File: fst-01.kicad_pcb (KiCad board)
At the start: 2 copper layers, 26.5 x 13.1 mm, 24 parts, among them J1 USB_A, K1 CONN_3, K2 CONN_2, K3 CONN_2, U1 STM32F103TB, U2 LP2985-33DBVR, U3 NUF2221W1, U4 SST25VF032B, X1 12MHz

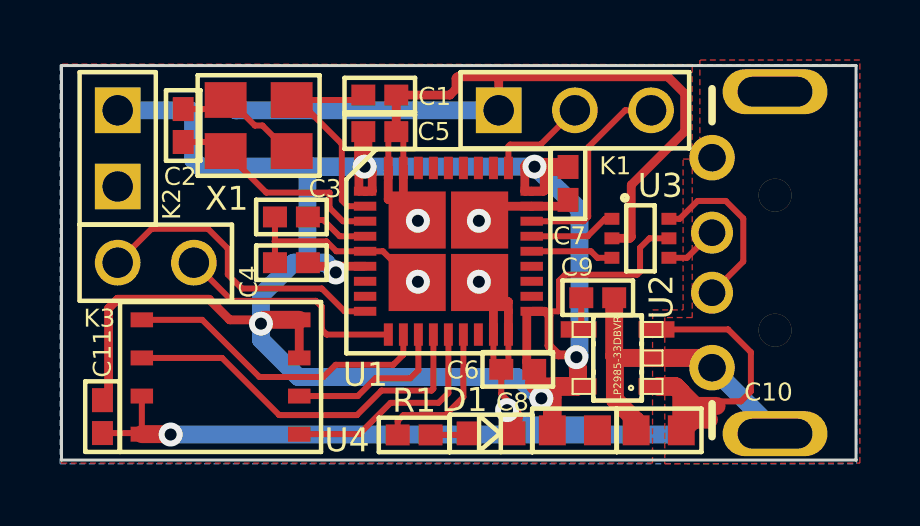
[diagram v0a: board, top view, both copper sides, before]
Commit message: update PCB
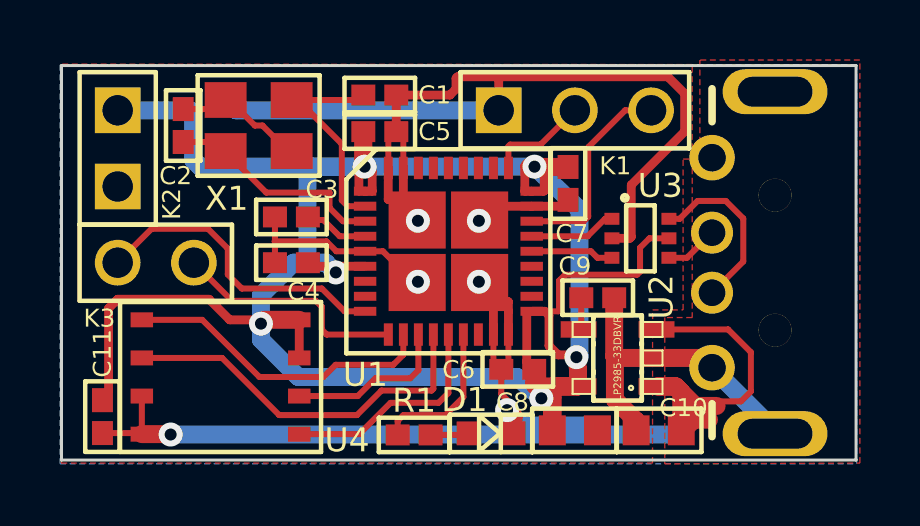
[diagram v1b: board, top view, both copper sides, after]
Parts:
- C1, C11, C2, C3, C4, C5, C6, C7, C9: footprint c_0402 -> FST:c_0402
- C10, C8: footprint c_0603 -> FST:c_0603
- R1: footprint r_0402 -> FST:r_0402
- X1: footprint ABM8G -> FST:ABM8G
